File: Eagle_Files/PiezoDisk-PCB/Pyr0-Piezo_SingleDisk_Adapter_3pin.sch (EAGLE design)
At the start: 4 parts, among them J1 C-GRID-03-70553

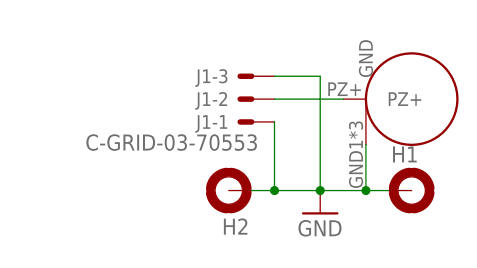
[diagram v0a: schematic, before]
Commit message: updated piezoPCB singledisk for better actuation #bugfix
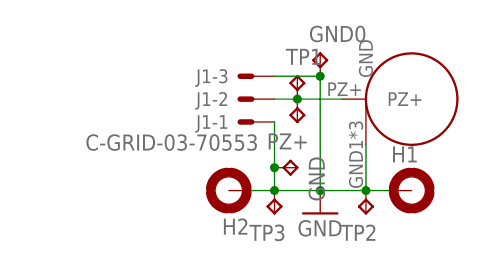
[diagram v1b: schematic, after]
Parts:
- added GND, GND0, PZ+: TPTP12SQ, PiezoFFC:TPTP12SQ
- added TP1, TP2, TP3: TPTP16R_LONG, PiezoFFC:TPTP16R_LONG
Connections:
- net GND: now also GND.TP, GND0.TP, TP2.TP, TP3.TP
- net PZ+: now also PZ+.TP, TP1.TP
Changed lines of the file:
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@@
 </classes>
 <parts>
-<part name="PZ1" library="PiezoFFC" library_urn="urn:adsk.eagle:library:6897166" deviceset="PIEZO-DISK" device="12MM-OFFSET" package3d_urn="urn:adsk.eagle:package:16537148/2" value="PIEZO-DISK12MM-OFFSET"/>
+<part name="PZ1" library="PiezoFFC" library_urn="urn:adsk.eagle:library:6897166" deviceset="PIEZO-DISK" device="12MM-OFFSET" package3d_urn="urn:adsk.eagle:package:16537148/3" value="PIEZO-DISK12MM-OFFSET"/>
 <part name="J1" library="PiezoFFC" library_urn="urn:adsk.eagle:library:6897166" deviceset="C-GRID-03" device="-70553" package3d_urn="urn:adsk.eagle:package:7346260/2"/>
 <part name="GND1" library="supply1" library_urn="urn:adsk.eagle:library:371" deviceset="GND" device=""/>
 <part name="H1" library="PiezoFFC" library_urn="urn:adsk.eagle:library:6897166" deviceset="HOLES_MOUNT-PAD-ROUND" device="3.2" package3d_urn="urn:adsk.eagle:package:5224590/3"/>
 <part name="H2" library="PiezoFFC" library_urn="urn:adsk.eagle:library:6897166" deviceset="HOLES_MOUNT-PAD-ROUND" device="3.2" package3d_urn="urn:adsk.eagle:package:5224590/3"/>
+<part name="GND0" library="PiezoFFC" library_urn="urn:adsk.eagle:library:6897166" deviceset="TP" device="TP12SQ" package3d_urn="urn:adsk.eagle:package:27964/1" value="TPTP12SQ"/>
+<part name="GND" library="PiezoFFC" library_urn="urn:adsk.eagle:library:6897166" deviceset="TP" device="TP12SQ" package3d_urn="urn:adsk.eagle:package:27964/1" value="TPTP12SQ"/>
+<part name="PZ+" library="PiezoFFC" library_urn="urn:adsk.eagle:library:6897166" deviceset="TP" device="TP12SQ" package3d_urn="urn:adsk.eagle:package:27964/1" value="TPTP12SQ"/>
+<part name="TP1" library="PiezoFFC" library_urn="urn:adsk.eagle:library:6897166" deviceset="TP" device="TP16R_LONG" package3d_urn="urn:adsk.eagle:package:16559598/1"/>
+<part name="TP2" library="PiezoFFC" library_urn="urn:adsk.eagle:library:6897166" deviceset="TP" device="TP16R_LONG" package3d_urn="urn:adsk.eagle:package:16559598/1"/>
+<part name="TP3" library="PiezoFFC" library_urn="urn:adsk.eagle:library:6897166" deviceset="TP" device="TP16R_LONG" package3d_urn="urn:adsk.eagle:package:16559598/1"/>
 </parts>
 <sheets>
@@
 <attribute name="NAME" x="-10.16" y="16.002" size="1.524" layer="95" rot="R180"/>
 </instance>
+<instance part="GND0" gate="G$1" x="0" y="17.78" smashed="yes">
+<attribute name="NAME" x="-1.27" y="19.05" size="1.778" layer="95"/>
+</instance>
+<instance part="GND" gate="G$1" x="-2.54" y="5.08" smashed="yes" rot="R270">
+<attribute name="NAME" x="-1.27" y="6.35" size="1.778" layer="95" rot="R270"/>
+</instance>
+<instance part="PZ+" gate="G$1" x="-2.54" y="10.16" smashed="yes" rot="R180">
+<attribute name="NAME" x="-1.27" y="8.89" size="1.778" layer="95" rot="R180"/>
+</instance>
+<instance part="TP1" gate="G$1" x="-2.54" y="15.24" smashed="yes">
+<attribute name="NAME" x="-3.81" y="16.51" size="1.778" layer="95"/>
+</instance>
+<instance part="TP2" gate="G$1" x="5.08" y="0" smashed="yes" rot="R180">
+<attribute name="NAME" x="6.35" y="-1.27" size="1.778" layer="95" rot="R180"/>
+</instance>
+<instance part="TP3" gate="G$1" x="-5.08" y="0" smashed="yes" rot="R180">
+<attribute name="NAME" x="-3.81" y="-1.27" size="1.778" layer="95" rot="R180"/>
+</instance>
 </instances>
 <busses>
@@
 <pinref part="PZ1" gate="G$1" pin="PZ+"/>
 <pinref part="J1" gate="-2" pin="S"/>
-<wire x1="2.54" y1="12.7" x2="-5.08" y2="12.7" width="0.1524" layer="91"/>
+<wire x1="2.54" y1="12.7" x2="-2.54" y2="12.7" width="0.1524" layer="91"/>
+<pinref part="PZ+" gate="G$1" pin="TP"/>
+<wire x1="-2.54" y1="12.7" x2="-5.08" y2="12.7" width="0.1524" layer="91"/>
+<junction x="-2.54" y="12.7"/>
+<pinref part="TP1" gate="G$1" pin="TP"/>
 </segment>
 </net>
@@
 <segment>
 <pinref part="J1" gate="-1" pin="S"/>
-<wire x1="-5.08" y1="10.16" x2="-5.08" y2="2.54" width="0.1524" layer="91"/>
+<wire x1="-5.08" y1="10.16" x2="-5.08" y2="5.08" width="0.1524" layer="91"/>
+<wire x1="-5.08" y1="5.08" x2="-5.08" y2="2.54" width="0.1524" layer="91"/>
 <wire x1="-5.08" y1="2.54" x2="0" y2="2.54" width="0.1524" layer="91"/>
 <pinref part="PZ1" gate="G$1" pin="GND"/>
 <wire x1="0" y1="2.54" x2="5.08" y2="2.54" width="0.1524" layer="91"/>
-<wire x1="5.08" y1="2.54" x2="5.08" y2="7.62" width="0.1524" layer="91"/>
 <pinref part="GND1" gate="1" pin="GND"/>
 <junction x="0" y="2.54"/>
 <pinref part="H2" gate="G$1" pin="MOUNT"/>
+<wire x1="5.08" y1="2.54" x2="5.08" y2="7.62" width="0.1524" layer="91"/>
 <wire x1="-7.62" y1="2.54" x2="-5.08" y2="2.54" width="0.1524" layer="91"/>
 <junction x="-5.08" y="2.54"/>
@@
 <wire x1="-5.08" y1="15.24" x2="0" y2="15.24" width="0.1524" layer="91"/>
 <wire x1="0" y1="15.24" x2="0" y2="2.54" width="0.1524" layer="91"/>
+<pinref part="GND0" gate="G$1" pin="TP"/>
+<junction x="0" y="15.24"/>
+<pinref part="GND" gate="G$1" pin="TP"/>
+<junction x="-5.08" y="5.08"/>
+<pinref part="TP2" gate="G$1" pin="TP"/>
+<pinref part="TP3" gate="G$1" pin="TP"/>
 </segment>
 </net>
